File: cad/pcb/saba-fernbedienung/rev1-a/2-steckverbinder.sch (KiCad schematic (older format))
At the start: 29 parts, among them J301 Conn_01x04, J302 Conn_01x04, J303 Micro_SD_Card, J304 Conn_01x04, J305 AudioJack3, J306 Conn_01x02, J307 Conn_01x04, J308 Conn_01x01, J309 Conn_01x01, J310 Conn_01x01, J311 Conn_01x04, J312 Conn_01x08, J313 USB_C_Receptacle_USB2.0, U301 TSOP31238

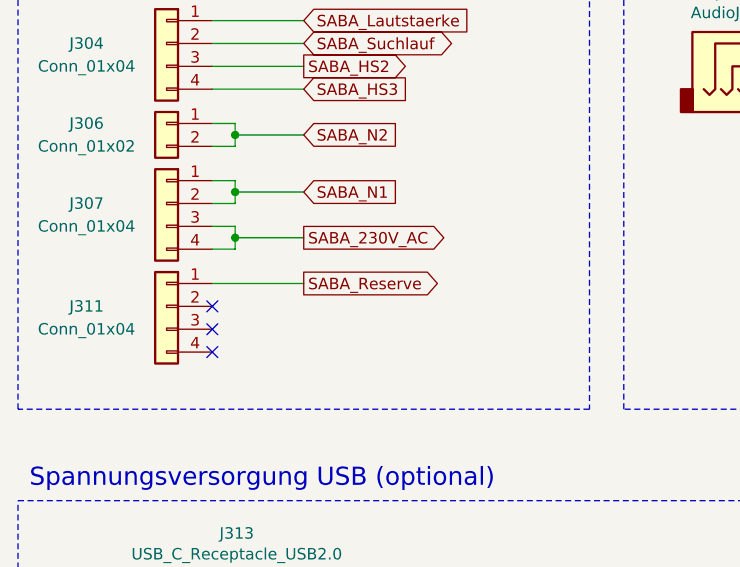
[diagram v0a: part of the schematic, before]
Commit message: Sicherung
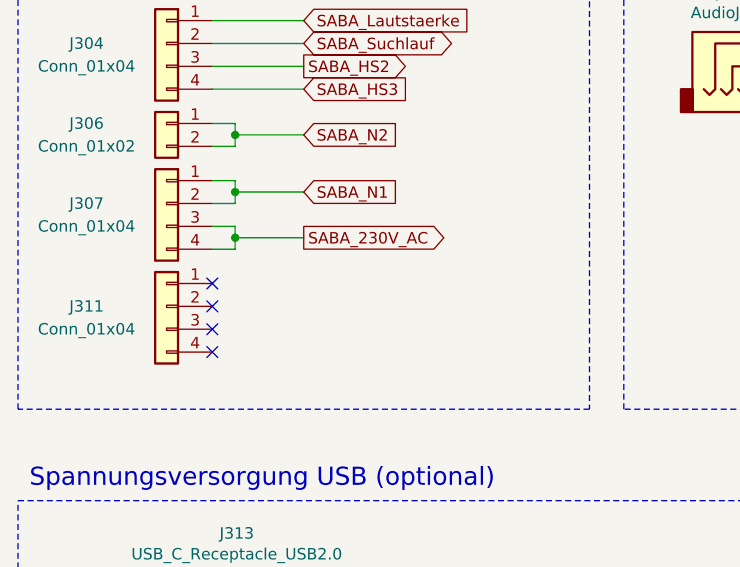
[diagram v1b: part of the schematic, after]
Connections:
- net SABA_Reserve: no longer names the net of J311.1 (Pin_1)
- no-connect marks 11 -> 12
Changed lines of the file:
@@
 	4450 3100 4450 2600
 Connection ~ 4450 2600
-Text GLabel 2250 3200 2    50   Output ~ 0
-SABA_Reserve
-Wire Wire Line
-	2250 3200 1850 3200
 $Comp
 L Connector_Generic:Conn_01x08 J312
@@
 	1    0    0    -1
 $EndComp
+NoConn ~ 1850 3200
 $EndSCHEMATC

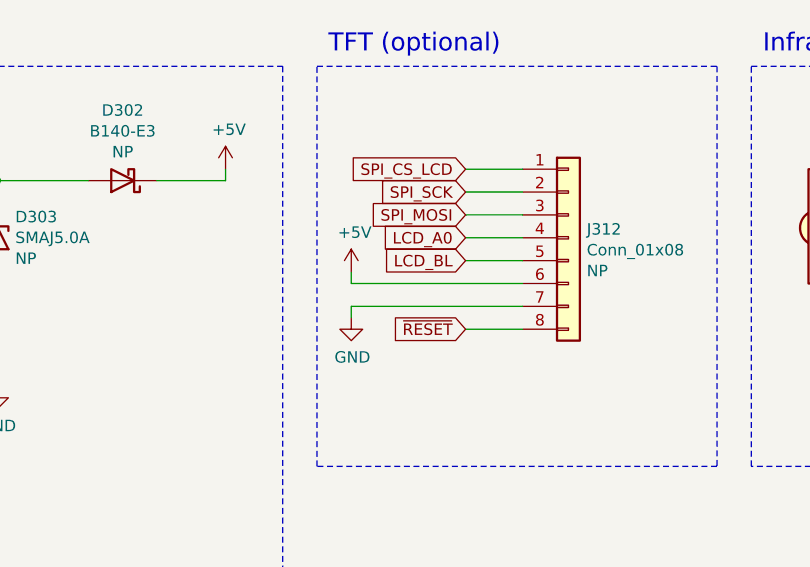
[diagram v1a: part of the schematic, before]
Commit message: Sicherung
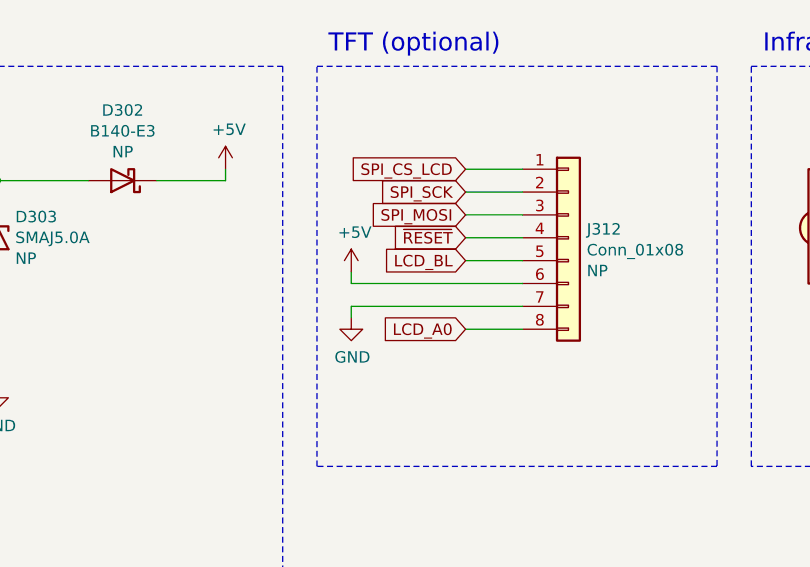
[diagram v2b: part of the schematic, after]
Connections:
- net LCD_A0: now also J312.8 (Pin_8); no longer J312.4 (Pin_4)
- net ~RESET: now also J312.4 (Pin_4); no longer J312.8 (Pin_8)
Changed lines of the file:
@@
 Text GLabel 6150 4800 0    50   Input ~ 0
 SPI_MOSI
+Text GLabel 6150 4900 0    50   Input ~ 0
+~RESET
 Text GLabel 6150 5300 0    50   Input ~ 0
-~RESET
-Text GLabel 6150 4900 0    50   Input ~ 0
 LCD_A0
 Text GLabel 6150 5000 0    50   Input ~ 0
